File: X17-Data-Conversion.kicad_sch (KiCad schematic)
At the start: 18 parts, among them J1 Conn_01x05, J4 Conn_01x12_Pin, U2 STM32F091CCTx, U4 MAX7375AXR805+T, U5 AZ1117IH-3.3TRG1

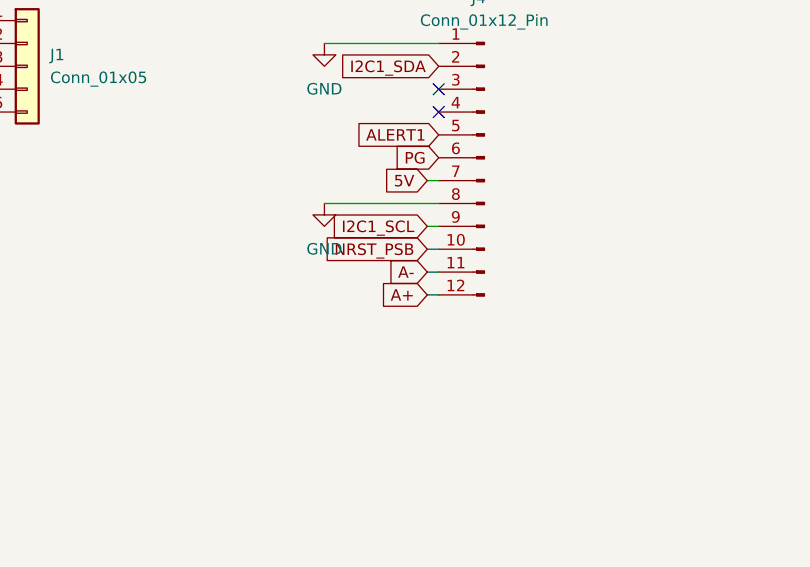
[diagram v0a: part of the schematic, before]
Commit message: here ya go
here ya go
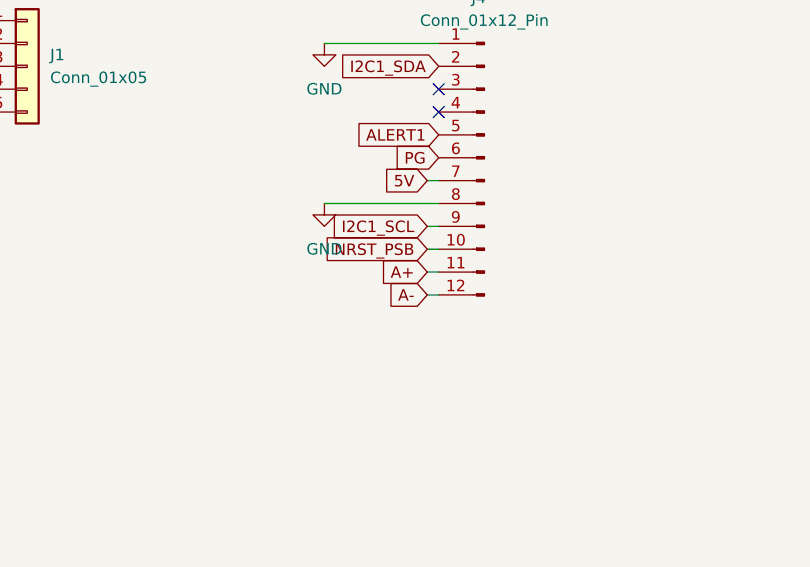
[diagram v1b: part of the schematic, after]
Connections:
- net A+: now also J4.11 (Pin_11); no longer J4.12 (Pin_12)
- net A-: now also J4.12 (Pin_12); no longer J4.11 (Pin_11)
